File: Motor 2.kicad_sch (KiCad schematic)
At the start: 25 parts, among them IC3 BTS7960B, IC4 BTS7960B, U5 HCPL-2630

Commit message: layout v2
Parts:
- C10, C11, C15, C16, C3, C7: footprint Capacitor_SMD:C_0805_2012Metric_Pad1.18x1.45mm_HandSolder -> Capacitor_SMD:C_0603_1608Metric_Pad1.08x0.95mm_HandSolder
- R10, R11, R12, R13, R14, R15, R16, R29, R30, R31, R32, R9: footprint Resistor_SMD:R_0805_2012Metric_Pad1.20x1.40mm_HandSolder -> Resistor_SMD:R_0603_1608Metric_Pad0.98x0.95mm_HandSolder
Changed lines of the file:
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@@
 			)
 		)
-		(property "Footprint" "Resistor_SMD:R_0805_2012Metric_Pad1.20x1.40mm_HandSolder"
+		(property "Footprint" "Resistor_SMD:R_0603_1608Metric_Pad0.98x0.95mm_HandSolder"
 			(at 94.488 96.52 90)
 			(hide yes)
@@
 			)
 		)
-		(property "Footprint" "Resistor_SMD:R_0805_2012Metric_Pad1.20x1.40mm_HandSolder"
+		(property "Footprint" "Resistor_SMD:R_0603_1608Metric_Pad0.98x0.95mm_HandSolder"
 			(at 94.488 83.82 90)
 			(hide yes)
@@
 			)
 		)
-		(property "Footprint" "Capacitor_SMD:C_0805_2012Metric_Pad1.18x1.45mm_HandSolder"
+		(property "Footprint" "Capacitor_SMD:C_0603_1608Metric_Pad1.08x0.95mm_HandSolder"
 			(at 115.2652 115.57 0)
 			(hide yes)
@@
 			)
 		)
-		(property "Footprint" "Resistor_SMD:R_0805_2012Metric_Pad1.20x1.40mm_HandSolder"
+		(property "Footprint" "Resistor_SMD:R_0603_1608Metric_Pad0.98x0.95mm_HandSolder"
 			(at 195.072 86.36 90)
 			(hide yes)
@@
 			)
 		)
-		(property "Footprint" "Resistor_SMD:R_0805_2012Metric_Pad1.20x1.40mm_HandSolder"
+		(property "Footprint" "Resistor_SMD:R_0603_1608Metric_Pad0.98x0.95mm_HandSolder"
 			(at 106.172 111.76 90)
 			(hide yes)
@@
 			)
 		)
-		(property "Footprint" "Capacitor_SMD:C_0805_2012Metric_Pad1.18x1.45mm_HandSolder"
+		(property "Footprint" "Capacitor_SMD:C_0603_1608Metric_Pad1.08x0.95mm_HandSolder"
 			(at 199.0852 130.81 0)
 			(hide yes)
@@
 			)
 		)
-		(property "Footprint" "Resistor_SMD:R_0805_2012Metric_Pad1.20x1.40mm_HandSolder"
+		(property "Footprint" "Resistor_SMD:R_0603_1608Metric_Pad0.98x0.95mm_HandSolder"
 			(at 62.23 94.742 90)
 			(hide yes)
@@
 			)
 		)
-		(property "Footprint" "Capacitor_SMD:C_0805_2012Metric_Pad1.18x1.45mm_HandSolder"
+		(property "Footprint" "Capacitor_SMD:C_0603_1608Metric_Pad1.08x0.95mm_HandSolder"
 			(at 148.2852 129.54 0)
 			(hide yes)
@@
 			)
 		)
-		(property "Footprint" "Capacitor_SMD:C_0805_2012Metric_Pad1.18x1.45mm_HandSolder"
+		(property "Footprint" "Capacitor_SMD:C_0603_1608Metric_Pad1.08x0.95mm_HandSolder"
 			(at 197.8152 113.03 0)
 			(hide yes)
@@
 			)
 		)
-		(property "Footprint" "Resistor_SMD:R_0805_2012Metric_Pad1.20x1.40mm_HandSolder"
+		(property "Footprint" "Resistor_SMD:R_0603_1608Metric_Pad0.98x0.95mm_HandSolder"
 			(at 62.23 89.662 90)
 			(hide yes)
@@
 			)
 		)
-		(property "Footprint" "Resistor_SMD:R_0805_2012Metric_Pad1.20x1.40mm_HandSolder"
+		(property "Footprint" "Resistor_SMD:R_0603_1608Metric_Pad0.98x0.95mm_HandSolder"
 			(at 202.692 109.22 90)
 			(hide yes)
@@
 			)
 		)
-		(property "Footprint" "Capacitor_SMD:C_0805_2012Metric_Pad1.18x1.45mm_HandSolder"
+		(property "Footprint" "Capacitor_SMD:C_0603_1608Metric_Pad1.08x0.95mm_HandSolder"
 			(at 127.9652 115.57 0)
 			(hide yes)
@@
 			)
 		)
-		(property "Footprint" "Capacitor_SMD:C_0805_2012Metric_Pad1.18x1.45mm_HandSolder"
+		(property "Footprint" "Capacitor_SMD:C_0603_1608Metric_Pad1.08x0.95mm_HandSolder"
 			(at 185.1152 113.03 0)
 			(hide yes)
@@
 			)
 		)
-		(property "Footprint" "Resistor_SMD:R_0805_2012Metric_Pad1.20x1.40mm_HandSolder"
+		(property "Footprint" "Resistor_SMD:R_0603_1608Metric_Pad0.98x0.95mm_HandSolder"
 			(at 131.572 86.36 90)
 			(hide yes)
@@
 			)
 		)
-		(property "Footprint" "Resistor_SMD:R_0805_2012Metric_Pad1.20x1.40mm_HandSolder"
+		(property "Footprint" "Resistor_SMD:R_0603_1608Metric_Pad0.98x0.95mm_HandSolder"
 			(at 120.142 86.36 90)
 			(hide yes)
@@
 			)
 		)
-		(property "Footprint" "Resistor_SMD:R_0805_2012Metric_Pad1.20x1.40mm_HandSolder"
+		(property "Footprint" "Resistor_SMD:R_0603_1608Metric_Pad0.98x0.95mm_HandSolder"
 			(at 173.482 109.22 90)
 			(hide yes)
@@
 			)
 		)
-		(property "Footprint" "Resistor_SMD:R_0805_2012Metric_Pad1.20x1.40mm_HandSolder"
+		(property "Footprint" "Resistor_SMD:R_0603_1608Metric_Pad0.98x0.95mm_HandSolder"
 			(at 132.842 111.76 90)
 			(hide yes)
@@
 			)
 		)
-		(property "Footprint" "Resistor_SMD:R_0805_2012Metric_Pad1.20x1.40mm_HandSolder"
+		(property "Footprint" "Resistor_SMD:R_0603_1608Metric_Pad0.98x0.95mm_HandSolder"
 			(at 202.692 86.36 90)
 			(hide yes)

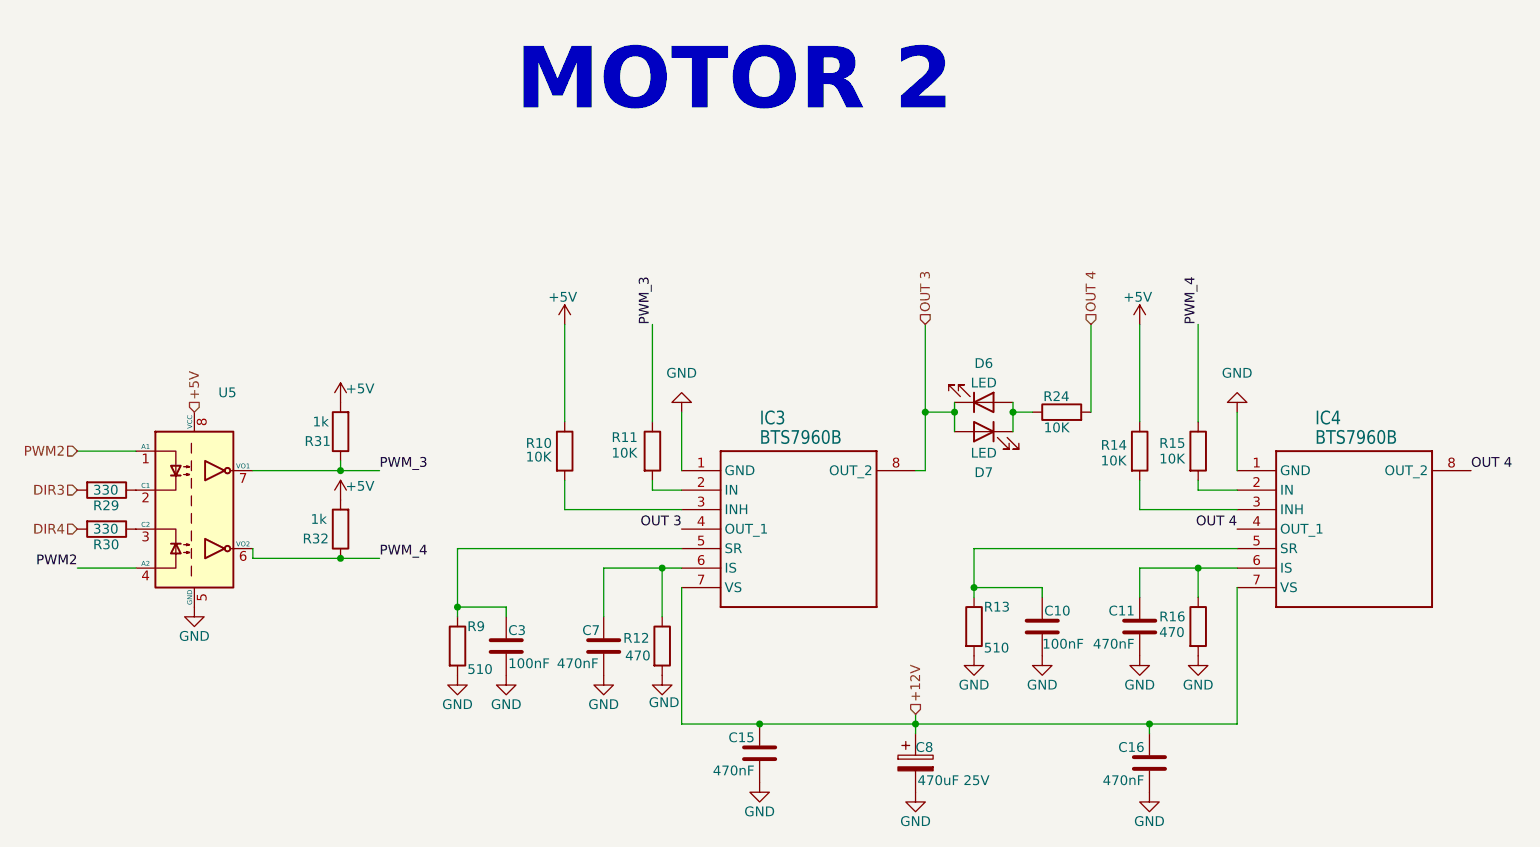
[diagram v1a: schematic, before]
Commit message: layout final v6
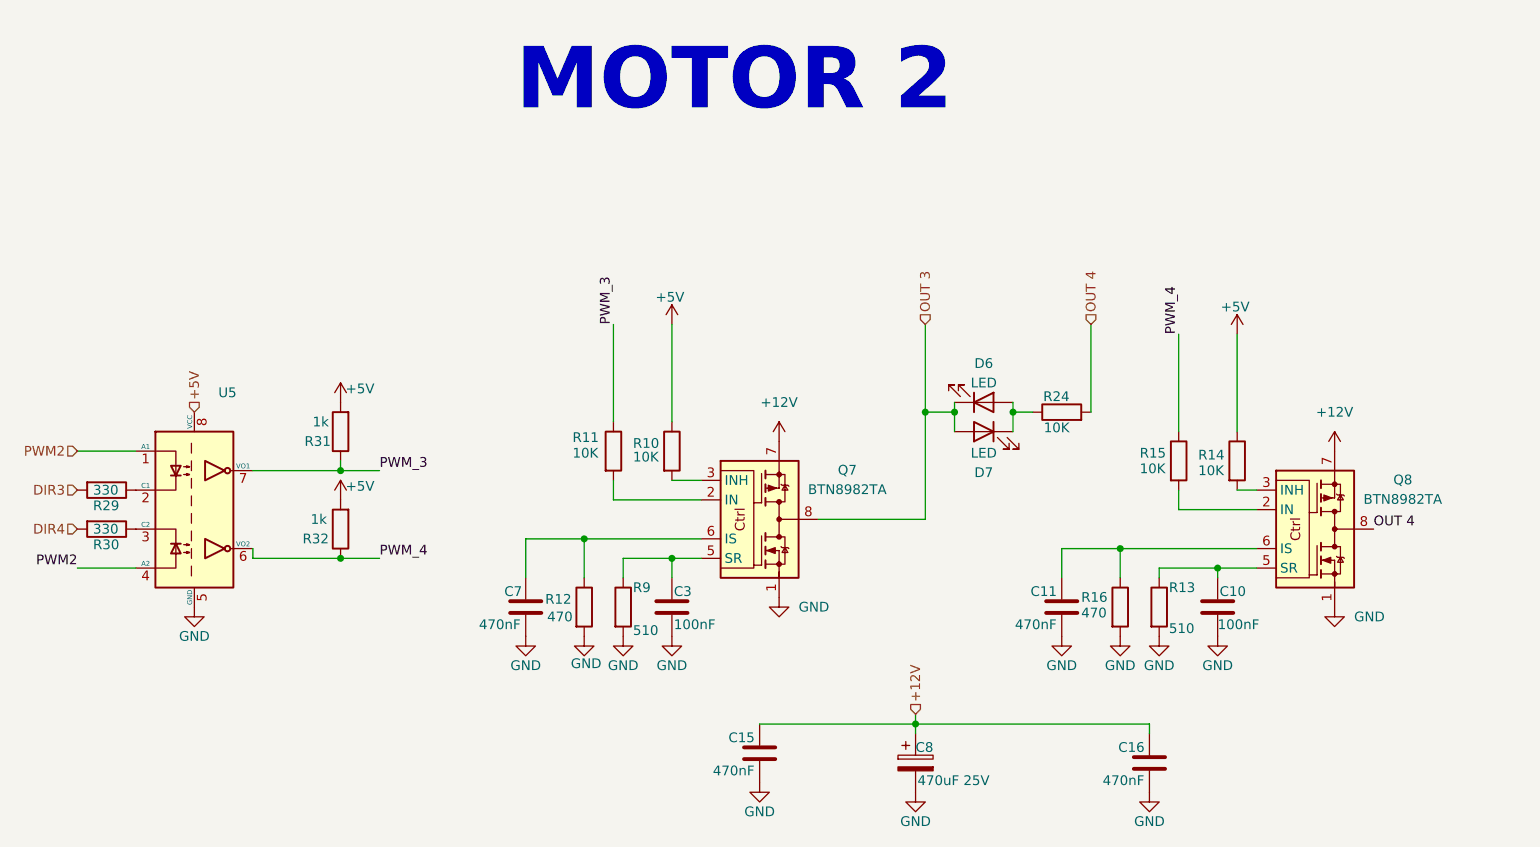
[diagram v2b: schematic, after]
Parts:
- removed IC3, IC4: BTS7960B, Package_TO_SOT_SMD:TO-263-7_TabPin8, symbol Driver BTN 2023 FIX-eagle-import:BTS7960B
- added Q7, Q8: BTN8982TA, Package_TO_SOT_SMD:TO-263-7_TabPin8, symbol Power_Management:BTN8982TA
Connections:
- net +12V: now also Q7.7, Q8.7
- net GND: now also Q7.1, Q8.1
- net OUT 3: now also Q7.4, Q7.8
- net OUT 4: now also Q8.4, Q8.8
- net at R15.2: now also Q8.2 (IN)
- net at R14.2: now also Q8.3 (INH)
- net at C10.1, R13.1: now also Q8.5 (SR)
- net at C11.1, R16.1: now also Q8.6 (IS)
- net at C3.1, R9.1: now also Q7.5 (SR)
- net at C7.1, R12.1: now also Q7.6 (IS)
- net at R11.2: now also Q7.2 (IN)
- net at R10.2: now also Q7.3 (INH)
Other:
- moved on the sheet: C10, C11, C3, C7, R10, R11, R12, R13, R14, R15, R16, R9
